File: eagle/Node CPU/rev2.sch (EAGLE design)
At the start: 44 parts, among them IC1 MEGA8-AI

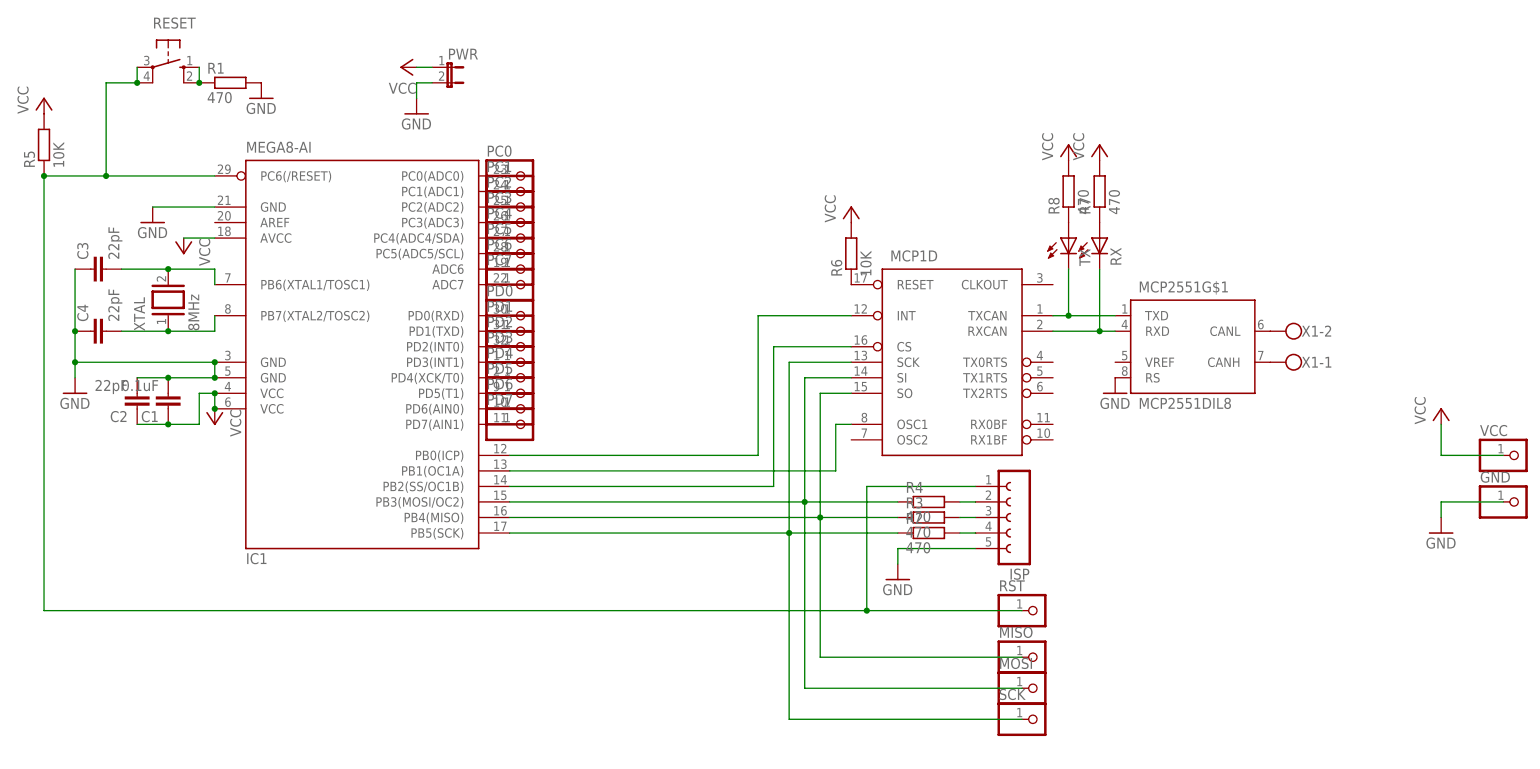
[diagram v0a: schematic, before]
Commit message: updated to revision 3 of the board
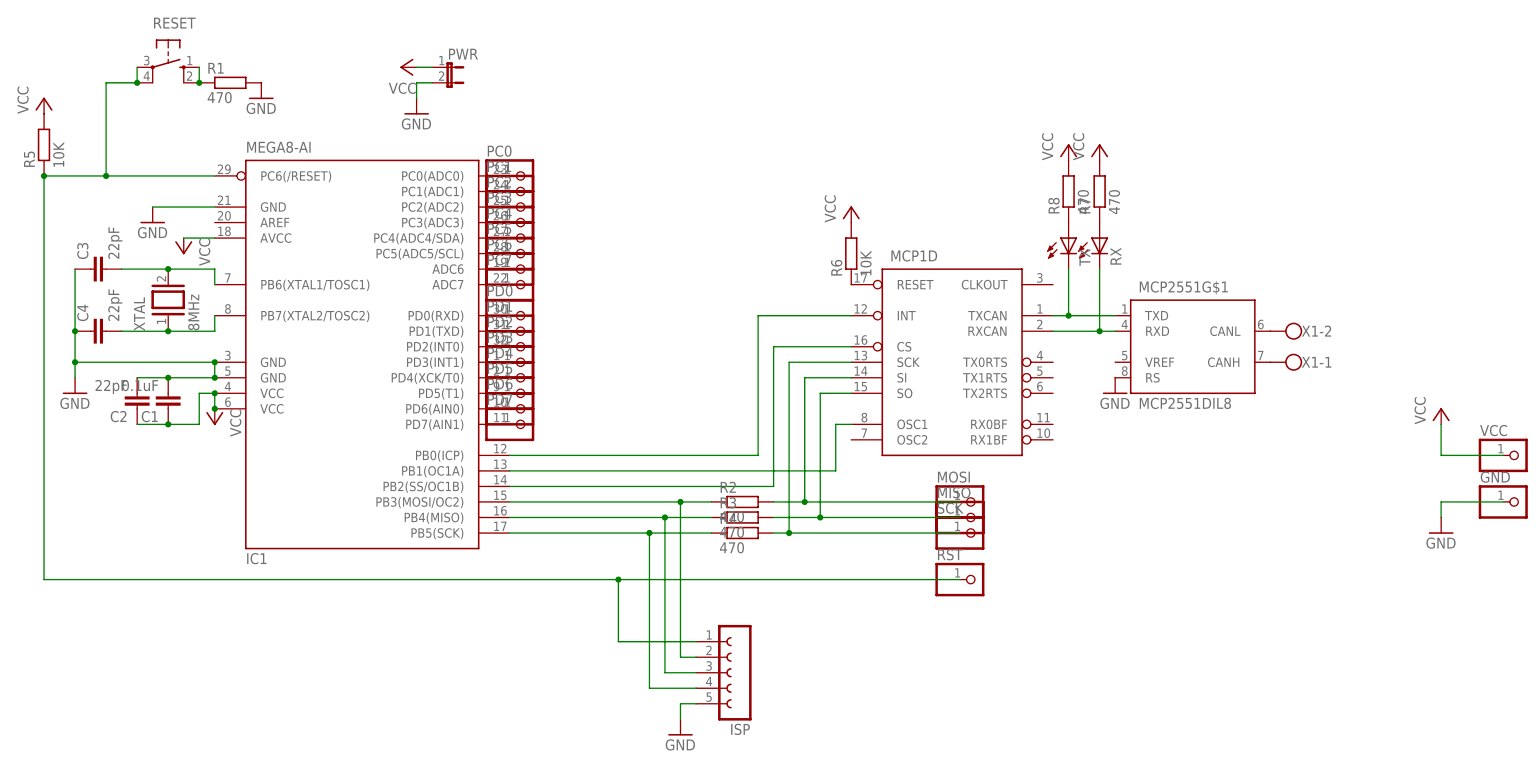
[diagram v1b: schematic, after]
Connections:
- removed net N$1: IC1.PB5(SCK), MCP1D.SCK, R2.1, SCK.1
- removed net N$16: ISP.3, R3.2
- new net N$38: MCP1D.SO, MISO.1, R3.2
- new net N$39: IC1.PB5(SCK), ISP.4, R4.1
- net N$15: now also MCP1D.SCK, SCK.1; no longer ISP.2
- net N$17: now also IC1.PB3(MOSI/OC2), ISP.2, R2.1; no longer ISP.4, R2.2
- net N$2: now also ISP.3; no longer MCP1D.SO, MISO.1
- net N$3: now also R2.2; no longer IC1.PB3(MOSI/OC2), R4.1
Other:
- moved on the sheet: ISP, MISO, MOSI, R2, R3, R4, RST, SCK
